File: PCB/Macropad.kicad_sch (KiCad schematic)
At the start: 9 parts, among them SW1 SW_Push, SW2 SW_Push, SW3 SW_Push, SW4 SW_Push, SW5 SW_Push, SW6 SW_Push, U1 XIAO-RP2040-DIP

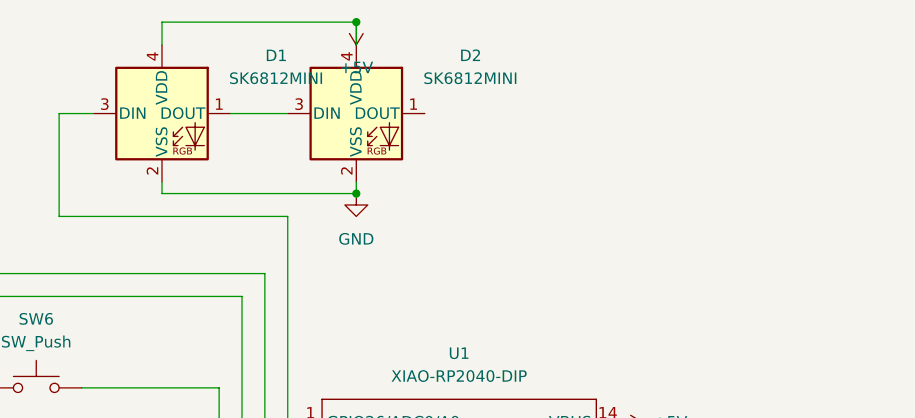
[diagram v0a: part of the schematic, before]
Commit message: edited
edited
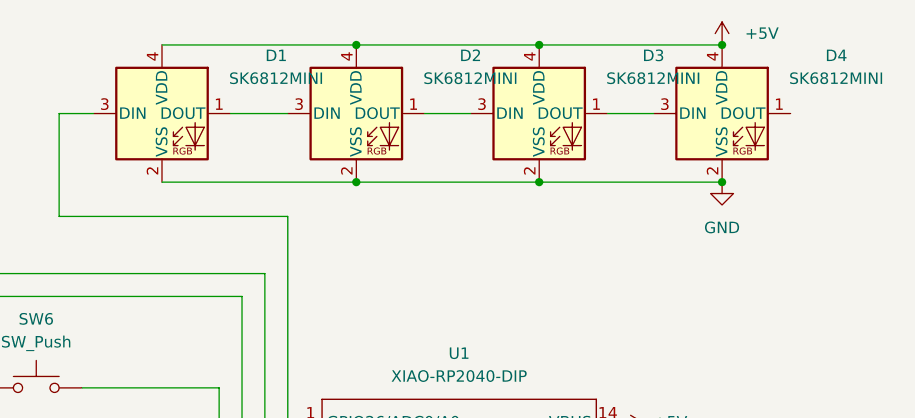
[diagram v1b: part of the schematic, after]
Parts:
- added D3, D4: SK6812MINI, LED_SMD:LED_SK6812MINI_PLCC4_3.5x3.5mm_P1.75mm, symbol LED:SK6812MINI
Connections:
- net +5V: now also D3.4 (VDD), D4.4 (VDD)
- net GND: now also D3.2 (VSS), D4.2 (VSS)
- net at D2.1 (DOUT): now also D3.3 (DIN)
- new net: D3.1 (DOUT), D4.3 (DIN)
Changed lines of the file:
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@@
+	)
+	(junction
+		(at 134.62 52.07)
+		(diameter 0)
+		(color 0 0 0 0)
 	)
 	(junction
@@
 	)
 	(junction
-		(at 93.98 68.58)
+		(at 93.98 67.31)
 		(diameter 0)
 		(color 0 0 0 0)
@@
 	)
 	(junction
-		(at 93.98 49.53)
+		(at 114.3 67.31)
+		(diameter 0)
+		(color 0 0 0 0)
+	)
+	(junction
+		(at 93.98 52.07)
+		(diameter 0)
+		(color 0 0 0 0)
+	)
+	(junction
+		(at 134.62 67.31)
 		(diameter 0)
 		(color 0 0 0 0)
@@
 		(color 0 0 0 0)
 	)
+	(junction
+		(at 114.3 52.07)
+		(diameter 0)
+		(color 0 0 0 0)
+	)
 	(wire
 		(pts
@@
 	(wire
 		(pts
+			(xy 114.3 52.07) (xy 134.62 52.07)
+		)
+		(stroke
+			(width 0)
+			(type default)
+		)
+	)
+	(wire
+		(pts
 			(xy 63.5 128.27) (xy 74.93 128.27)
 		)
@@
 	(wire
 		(pts
-			(xy 72.39 67.31) (xy 72.39 68.58)
-		)
-		(stroke
-			(width 0)
-			(type default)
-		)
-	)
-	(wire
-		(pts
 			(xy 72.39 160.02) (xy 72.39 139.7)
 		)
@@
 	(wire
 		(pts
+			(xy 101.6 59.69) (xy 106.68 59.69)
+		)
+		(stroke
+			(width 0)
+			(type default)
+		)
+	)
+	(wire
+		(pts
 			(xy 83.82 77.47) (xy 45.72 77.47)
 		)
@@
 	(wire
 		(pts
+			(xy 72.39 52.07) (xy 93.98 52.07)
+		)
+		(stroke
+			(width 0)
+			(type default)
+		)
+	)
+	(wire
+		(pts
 			(xy 77.47 127) (xy 132.08 127)
 		)
@@
 	(wire
 		(pts
-			(xy 72.39 52.07) (xy 72.39 49.53)
-		)
-		(stroke
-			(width 0)
-			(type default)
-		)
-	)
-	(wire
-		(pts
 			(xy 81.28 80.01) (xy 81.28 116.84)
 		)
@@
 	(wire
 		(pts
+			(xy 93.98 67.31) (xy 114.3 67.31)
+		)
+		(stroke
+			(width 0)
+			(type default)
+		)
+	)
+	(wire
+		(pts
 			(xy 53.34 90.17) (xy 53.34 102.87)
 		)
@@
 	(wire
 		(pts
-			(xy 93.98 67.31) (xy 93.98 68.58)
-		)
-		(stroke
-			(width 0)
-			(type default)
-		)
-	)
-	(wire
-		(pts
 			(xy 135.89 129.54) (xy 135.89 105.41)
 		)
@@
 	(wire
 		(pts
+			(xy 93.98 52.07) (xy 114.3 52.07)
+		)
+		(stroke
+			(width 0)
+			(type default)
+		)
+	)
+	(wire
+		(pts
 			(xy 72.39 139.7) (xy 63.5 139.7)
 		)
@@
 	(wire
 		(pts
-			(xy 72.39 49.53) (xy 93.98 49.53)
-		)
-		(stroke
-			(width 0)
-			(type default)
-		)
-	)
-	(wire
-		(pts
 			(xy 123.19 109.22) (xy 133.35 109.22)
 		)
@@
 	(wire
 		(pts
-			(xy 72.39 68.58) (xy 93.98 68.58)
+			(xy 72.39 67.31) (xy 93.98 67.31)
+		)
+		(stroke
+			(width 0)
+			(type default)
+		)
+	)
+	(wire
+		(pts
+			(xy 114.3 67.31) (xy 134.62 67.31)
 		)
 		(stroke
@@
 	(wire
 		(pts
+			(xy 121.92 59.69) (xy 127 59.69)
+		)
+		(stroke
+			(width 0)
+			(type default)
+		)
+	)
+	(wire
+		(pts
 			(xy 53.34 151.13) (xy 53.34 152.4)
 		)
@@
 		(pts
 			(xy 60.96 59.69) (xy 64.77 59.69)
-		)
-		(stroke
-			(width 0)
-			(type default)
-		)
-	)
-	(wire
-		(pts
-			(xy 93.98 49.53) (xy 93.98 52.07)
 		)
 		(stroke
@@
 	)
 	(symbol
+		(lib_id "LED:SK6812MINI")
+		(at 134.62 59.69 0)
+		(unit 1)
+		(exclude_from_sim no)
+		(in_bom yes)
+		(on_board yes)
+		(dnp no)
+		(fields_autoplaced yes)
+		(property "Reference" "D4"
+			(at 147.32 53.2698 0)
+			(effects
+				(font
+					(size 1.27 1.27)
+				)
+			)
+		)
+		(property "Value" "SK6812MINI"
+			(at 147.32 55.8098 0)
+			(effects
+				(font
+					(size 1.27 1.27)
+				)
+			)
+		)
+		(property "Footprint" "LED_SMD:LED_SK6812MINI_PLCC4_3.5x3.5mm_P1.75mm"
+			(at 135.89 67.31 0)
+			(effects
+				(font
+					(size 1.27 1.27)
+				)
+				(justify left top)
+				(hide yes)
+			)
+		)
+		(property "Datasheet" "https://cdn-shop.adafruit.com/product-files/2686/SK6812MINI_REV.01-1-2.pdf"
+			(at 137.16 69.215 0)
+			(effects
+				(font
+					(size 1.27 1.27)
+				)
+				(justify left top)
+				(hide yes)
+			)
+		)
+		(property "Description" "RGB LED with integrated controller"
+			(at 134.62 59.69 0)
+			(effects
+				(font
+					(size 1.27 1.27)
+				)
+				(hide yes)
+			)
+		)
+		(pin "3"
+		)
+		(pin "2"
+		)
+		(pin "1"
+		)
+		(pin "4"
+		)
+		(instances
+			(project "Macropad"
+				(path "/40666a77-c9aa-469e-a75d-20a25f630b14"
+					(reference "D4")
+					(unit 1)
+				)
+			)
+		)
+	)
+	(symbol
 		(lib_id "Switch:SW_Push")
 		(at 58.42 90.17 0)
@@
 	(symbol
 		(lib_id "power:+5V")
-		(at 93.98 49.53 180)
+		(at 134.62 52.07 0)
 		(unit 1)
 		(exclude_from_sim no)
@@
 		(fields_autoplaced yes)
 		(property "Reference" "#PWR04"
-			(at 93.98 45.72 0)
+			(at 134.62 55.88 0)
 			(effects
 				(font
@@
 		)
 		(property "Value" "+5V"
-			(at 93.98 54.61 0)
-			(effects
-				(font
-					(size 1.27 1.27)
-				)
+			(at 137.16 50.7999 0)
+			(effects
+				(font
+					(size 1.27 1.27)
+				)
+				(justify left)
 			)
 		)
 		(property "Footprint" ""
-			(at 93.98 49.53 0)
+			(at 134.62 52.07 0)
 			(effects
 				(font
@@
 		)
 		(property "Datasheet" ""
-			(at 93.98 49.53 0)
+			(at 134.62 52.07 0)
 			(effects
 				(font
@@
 		)
 		(property "Description" "Power symbol creates a global label with name \"+5V\""
-			(at 93.98 49.53 0)
+			(at 134.62 52.07 0)
 			(effects
 				(font
@@
 	)
 	(symbol
+		(lib_id "LED:SK6812MINI")
+		(at 114.3 59.69 0)
+		(unit 1)
+		(exclude_from_sim no)
+		(in_bom yes)
+		(on_board yes)
+		(dnp no)
+		(fields_autoplaced yes)
+		(property "Reference" "D3"
+			(at 127 53.2698 0)
+			(effects
+				(font
+					(size 1.27 1.27)
+				)
+			)
+		)
+		(property "Value" "SK6812MINI"
+			(at 127 55.8098 0)
+			(effects
+				(font
+					(size 1.27 1.27)
+				)
+			)
+		)
+		(property "Footprint" "LED_SMD:LED_SK6812MINI_PLCC4_3.5x3.5mm_P1.75mm"
+			(at 115.57 67.31 0)
+			(effects
+				(font
+					(size 1.27 1.27)
+				)
+				(justify left top)
+				(hide yes)
+			)
+		)
+		(property "Datasheet" "https://cdn-shop.adafruit.com/product-files/2686/SK6812MINI_REV.01-1-2.pdf"
+			(at 116.84 69.215 0)
+			(effects
+				(font
+					(size 1.27 1.27)
+				)
+				(justify left top)
+				(hide yes)
+			)
+		)
+		(property "Description" "RGB LED with integrated controller"
+			(at 114.3 59.69 0)
+			(effects
+				(font
+					(size 1.27 1.27)
+				)
+				(hide yes)
+			)
+		)
+		(pin "3"
+		)
+		(pin "2"
+		)
+		(pin "1"
+		)
+		(pin "4"
+		)
+		(instances
+			(project "Macropad"
+				(path "/40666a77-c9aa-469e-a75d-20a25f630b14"
+					(reference "D3")
+					(unit 1)
+				)
+			)
+		)
+	)
+	(symbol
 		(lib_id "power:GND")
-		(at 93.98 68.58 0)
+		(at 134.62 67.31 0)
 		(unit 1)
 		(exclude_from_sim no)
@@
 		(fields_autoplaced yes)
 		(property "Reference" "#PWR03"
-			(at 93.98 74.93 0)
+			(at 134.62 73.66 0)
 			(effects
 				(font
@@
 		)
 		(property "Value" "GND"
-			(at 93.98 73.66 0)
+			(at 134.62 72.39 0)
 			(effects
 				(font
@@
 		)
 		(property "Footprint" ""
-			(at 93.98 68.58 0)
+			(at 134.62 67.31 0)
 			(effects
 				(font
@@
 		)
 		(property "Datasheet" ""
-			(at 93.98 68.58 0)
+			(at 134.62 67.31 0)
 			(effects
 				(font
@@
 		)
 		(property "Description" "Power symbol creates a global label with name \"GND\" , ground"
-			(at 93.98 68.58 0)
-			(effects
-				(font
+			(at 134.62 67.31 0)
+			(effects
+				(font
